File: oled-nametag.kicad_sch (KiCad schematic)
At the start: 13 parts, among them J1 USB_C_Receptacle_USB2.0, J2 I2C, SW1 Power, SW2 BTN1, SW3 BTN2, SW4 BTN3

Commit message: Add missing LCSC partnumbers
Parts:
- SW1, SW2, SW3, SW4: LCSC (none) -> C963349
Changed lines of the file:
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@@
+      (effects (font (size 1.27 1.27)) hide)
+    )
+    (property "LCSC" "C963349" (at 123.19 128.27 0)
       (effects (font (size 1.27 1.27)) hide)
     )
@@
       (effects (font (size 1.27 1.27)) hide)
     )
+    (property "LCSC" "C963349" (at 123.19 110.49 0)
+      (effects (font (size 1.27 1.27)) hide)
+    )
     (pin "1")
     (pin "2")
@@
     )
     (property "Datasheet" "https://www.mouser.de/datasheet/2/307/en-b3u-3615.pdf" (at 132.08 45.72 0)
+      (effects (font (size 1.27 1.27)) hide)
+    )
+    (property "LCSC" "C963349" (at 137.16 45.72 90)
       (effects (font (size 1.27 1.27)) hide)
     )
@@
       (effects (font (size 1.27 1.27)) hide)
     )
+    (property "LCSC" "C963349" (at 123.19 119.38 0)
+      (effects (font (size 1.27 1.27)) hide)
+    )

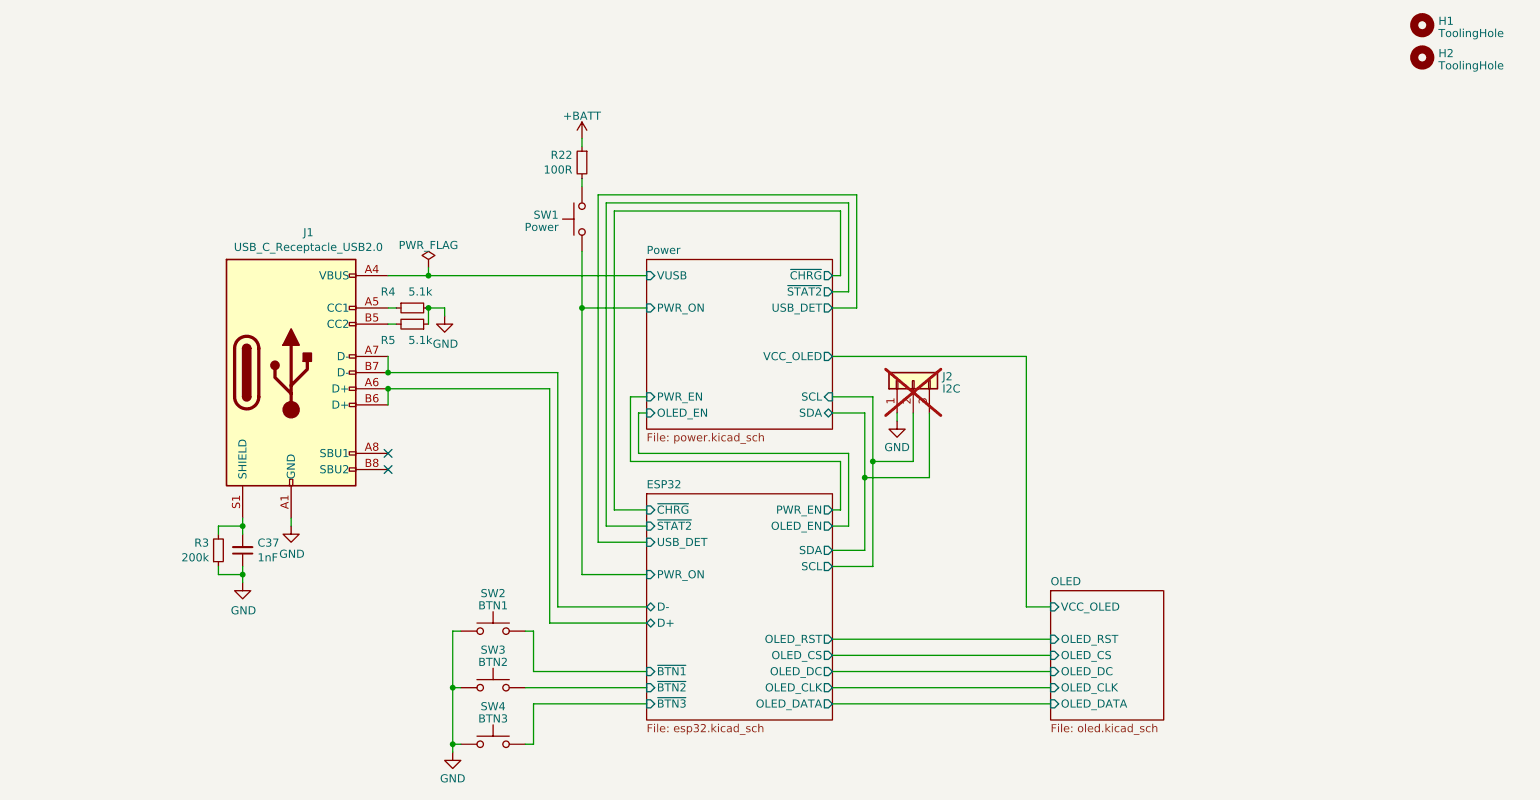
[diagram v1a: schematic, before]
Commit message: Finsh first layout iteration
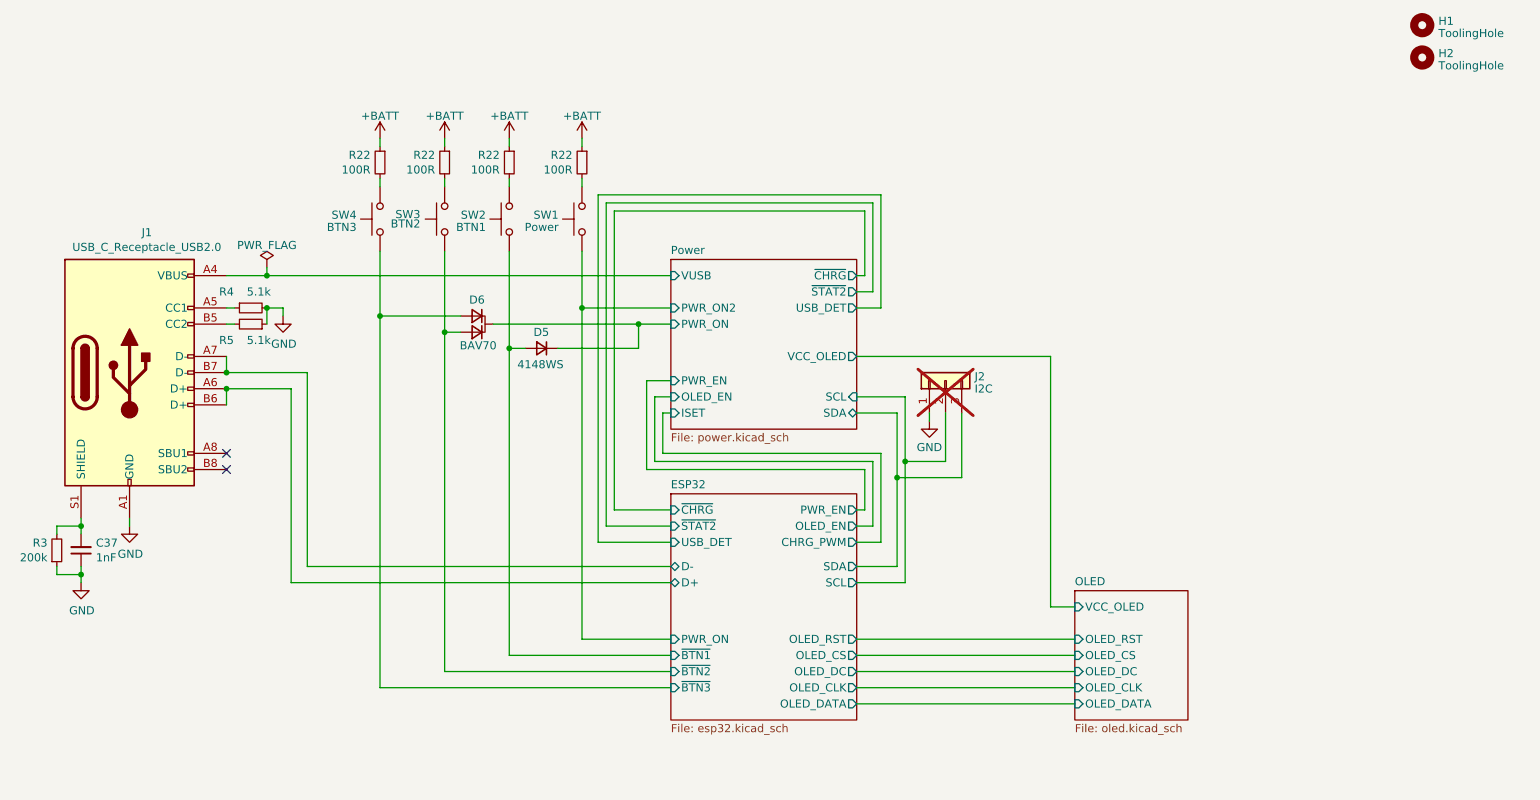
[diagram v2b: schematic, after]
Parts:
- added D5: 4148WS, Diode_SMD:D_SOD-323, symbol Device:D_Small
- added D6: BAV70, Package_TO_SOT_SMD:SOT-23, symbol BAV70_Small:BAV70_Small
- added R22 (x3): 100R, Resistor_SMD:R_0402_1005Metric, symbol Device:R_Small
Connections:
- net +BATT: now also R22.1, R22.1, R22.1
- net ESP32/~{BTN1}: now also D5.2 (A)
- net ESP32/~{BTN2}: now also SW3.1, D6.1 (A1); no longer SW3.2
- net ESP32/~{BTN3}: now also D6.2 (A2)
- net GND: no longer SW2.1, SW3.1, SW4.1
- new net: R22.2, SW4.1
- new net: R22.2, SW2.1
- new net: R22.2, SW3.2
- new net Power/PWR_ON: D5.1 (K), D6.3 (K)
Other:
- sheet ESP32 ports: added CHRG_PWM; removed none
- sheet Power ports: added ISET, PWR_ON2; removed none
- moved on the sheet: C37, J1, J2, R3, R4, R5, SW2, SW3, SW4
